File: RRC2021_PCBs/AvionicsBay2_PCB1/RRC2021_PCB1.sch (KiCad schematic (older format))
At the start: 15 parts, among them U1 ADXL357z, U2 MS5611, U3 BN220-GPS

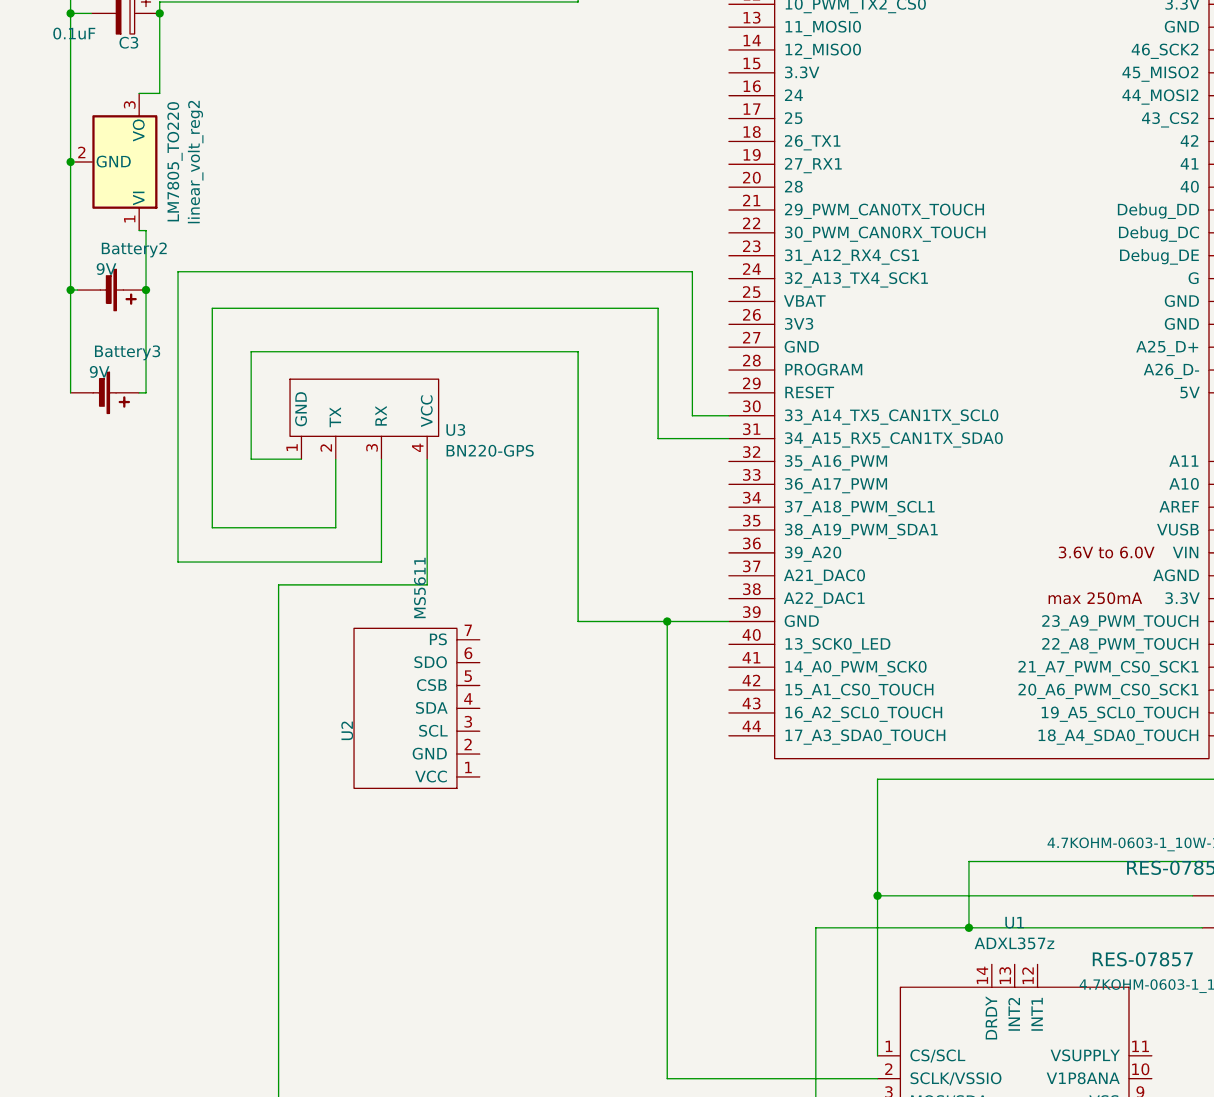
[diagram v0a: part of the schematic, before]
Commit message: update
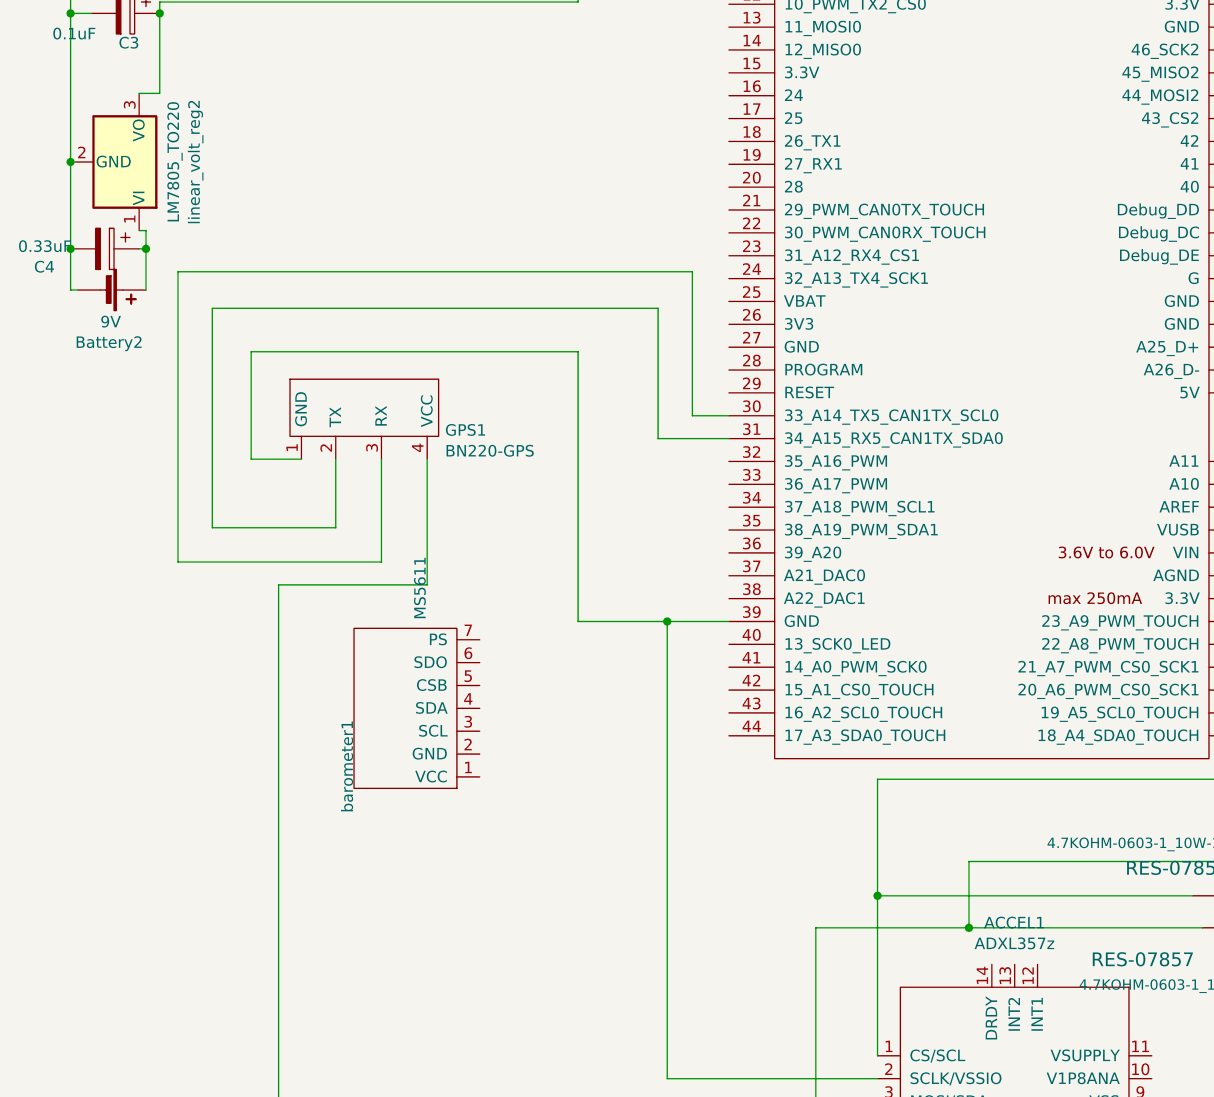
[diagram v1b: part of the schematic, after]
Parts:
- removed Battery3: 9V, Mounting Holes:1x02, symbol Device:Battery_Cell
- added C4: 0.33uF, Capacitor_SMD:CP_Elec_3x5.3, symbol Device:CP
- GPS1: renamed from U3; footprint Connector_PinSocket_2.54mm:PinSocket_1x04_P2.54mm_Vertical -> Connector_PinHeader_1.00mm:PinHeader_1x04_P1.00mm_Horizontal
- renumbered U1 to ACCEL1, U2 to barometer1
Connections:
- net at Battery2.2 (-), C3.2, RF1.2 (GND)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: now also C4.2
- net at Battery2.1 (+), linear_volt_reg2.1 (VI): now also C4.1
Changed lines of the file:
@@
 	8720 4530 8720 4880
 $Comp
-L RRC2021_PCB1-rescue:MS5611-RRC2021_PCB1-rescue U2
+L RRC2021_PCB1-rescue:MS5611-RRC2021_PCB1-rescue barometer1
 U 1 1 60AF376A
 P 2560 4560
-F 0 "U2" V 3038 5111 50  0000 L CNN
+F 0 "barometer1" V 3038 5111 50  0000 L CNN
 F 1 "MS5611" V 2720 4395 50  0000 L CNN
 F 2 "Mounting Holes:1x07" H 2560 4560 50  0001 C CNN
@@
 $EndComp
 $Comp
-L Device:Battery_Cell Battery3
-U 1 1 60F70EA5
-P 970 3680
-F 0 "Battery3" V 790 3680 50  0000 L CNN
-F 1 "9V" V 880 3660 50  0000 L CNN
-F 2 "Mounting Holes:1x02" V 970 3740 50  0001 C CNN
-F 3 "~" V 970 3740 50  0001 C CNN
-	1    970  3680
-	0    1    1    0
-$EndComp
-$Comp
 L Device:Battery_Cell Battery2
 U 1 1 60F724FD
 P 1000 3230
-F 0 "Battery2" V 820 3230 50  0000 L CNN
-F 1 "9V" V 910 3210 50  0000 L CNN
+F 0 "Battery2" V 1230 3120 50  0000 L CNN
+F 1 "9V" V 1140 3230 50  0000 L CNN
 F 2 "Mounting Holes:1x02" V 1000 3290 50  0001 C CNN
 F 3 "~" V 1000 3290 50  0001 C CNN
@@
 	960  2020 870  2020
 Wire Wire Line
-	1200 3230 1200 2970
-Wire Wire Line
 	1200 2970 1170 2970
 Wire Wire Line
 	900  3230 870  3230
-Wire Wire Line
-	870  3230 870  2670
 Connection ~ 870  2670
-Wire Wire Line
-	1170 3680 1200 3680
-Wire Wire Line
-	1200 3680 1200 3230
-Connection ~ 1200 3230
-Wire Wire Line
-	870  3680 870  3230
-Connection ~ 870  3230
 Wire Wire Line
 	6430 4880 8720 4880
@@
 	3750 1020 3750 980
 $Comp
-L RRC2021_PCB1-rescue:ADXL357z U1
+L RRC2021_PCB1-rescue:ADXL357z ACCEL1
 U 1 1 60B8F0A7
 P 4200 7280
-F 0 "U1" H 5000 8561 50  0000 C CNN
+F 0 "ACCEL1" H 5000 8561 50  0000 C CNN
 F 1 "ADXL357z" H 5000 8470 50  0000 C CNN
 F 2 "Mounting Holes:ADXLZ" H 5000 8580 50  0001 C CNN
@@
 Connection ~ 3480 4680
 $Comp
-L RRC2021_PCB1-rescue:BN220-GPS U3
+L RRC2021_PCB1-rescue:BN220-GPS GPS1
 U 1 1 60F710D4
 P 2130 3770
-F 0 "U3" H 2508 3696 50  0000 L CNN
+F 0 "GPS1" H 2508 3696 50  0000 L CNN
 F 1 "BN220-GPS" H 2508 3605 50  0000 L CNN
-F 2 "Connector_PinSocket_2.54mm:PinSocket_1x04_P2.54mm_Vertical" H 2130 3770 50  0001 C CNN
+F 2 "Connector_PinHeader_1.00mm:PinHeader_1x04_P1.00mm_Horizontal" H 2130 3770 50  0001 C CNN
 F 3 "" H 2130 3770 50  0001 C CNN
 	1    2130 3770
@@
 Wire Wire Line
 	2030 4270 2030 3970
+Wire Wire Line
+	870  2670 870  3050
+Wire Wire Line
+	1200 2970 1200 3050
+$Comp
+L Device:CP C4
+U 1 1 60F4269F
+P 1020 3050
+F 0 "C4" V 1100 2740 50  0000 L CNN
+F 1 "0.33uF" V 1010 2670 50  0000 L CNN
+F 2 "Capacitor_SMD:CP_Elec_3x5.3" H 1058 2900 50  0001 C CNN
+F 3 "~" H 1020 3050 50  0001 C CNN
+	1    1020 3050
+	0    1    1    0
+$EndComp
+Connection ~ 870  3050
+Wire Wire Line
+	870  3050 870  3230
+Wire Wire Line
+	1170 3050 1200 3050
+Connection ~ 1200 3050
+Wire Wire Line
+	1200 3050 1200 3230
 $EndSCHEMATC

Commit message: update
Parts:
- GPS1: footprint Connector_PinHeader_1.00mm:PinHeader_1x04_P1.00mm_Horizontal -> Connector_PinSocket_1.00mm:PinSocket_1x04_P1.00mm_Vertical
- R1, R2: footprint Resistors:0603 -> Resistor_THT:R_Axial_DIN0204_L3.6mm_D1.6mm_P5.08mm_Horizontal
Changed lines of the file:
@@
 F 0 "R1" H 5980 6180 45  0000 C CNN
 F 1 "4.7KOHM-0603-1_10W-1%" H 6410 5650 45  0000 C CNN
-F 2 "Resistors:0603" H 5980 6030 20  0001 C CNN
+F 2 "Resistor_THT:R_Axial_DIN0204_L3.6mm_D1.6mm_P5.08mm_Horizontal" H 5980 6030 20  0001 C CNN
 F 3 "" H 5980 5880 60  0001 C CNN
 F 4 "RES-07857" H 6250 5760 60  0000 C CNN "Field4"
@@
 F 0 "R2" H 6020 6320 45  0000 C CNN
 F 1 "4.7KOHM-0603-1_10W-1%" H 5690 5770 45  0000 C CNN
-F 2 "Resistors:0603" H 6020 6170 20  0001 C CNN
+F 2 "Resistor_THT:R_Axial_DIN0204_L3.6mm_D1.6mm_P5.08mm_Horizontal" H 6020 6170 20  0001 C CNN
 F 3 "" H 6020 6020 60  0001 C CNN
 F 4 "RES-07857" H 5560 5880 60  0000 C CNN "Field4"
@@
 F 0 "GPS1" H 2508 3696 50  0000 L CNN
 F 1 "BN220-GPS" H 2508 3605 50  0000 L CNN
-F 2 "Connector_PinHeader_1.00mm:PinHeader_1x04_P1.00mm_Horizontal" H 2130 3770 50  0001 C CNN
+F 2 "Connector_PinSocket_1.00mm:PinSocket_1x04_P1.00mm_Vertical" H 2130 3770 50  0001 C CNN
 F 3 "" H 2130 3770 50  0001 C CNN
 	1    2130 3770
